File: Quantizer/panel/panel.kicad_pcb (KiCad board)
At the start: 2 copper layers, 50.8 x 128.5 mm, 13 parts

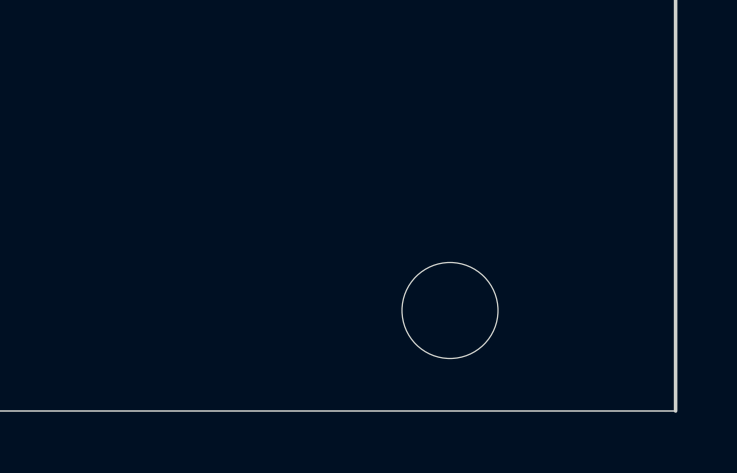
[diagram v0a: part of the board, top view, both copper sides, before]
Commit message: First commit
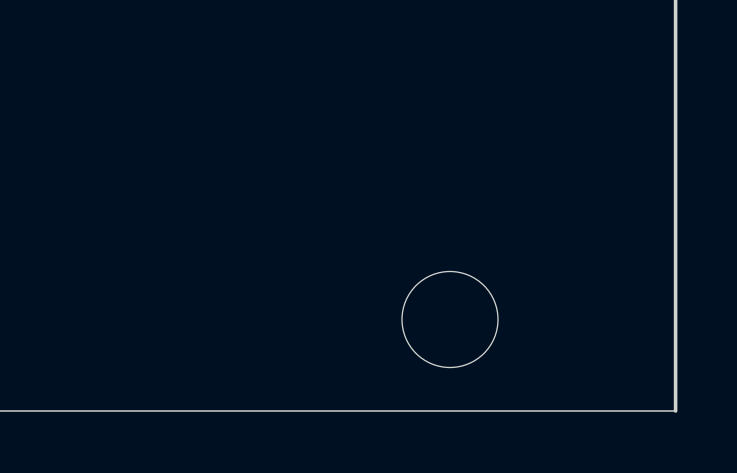
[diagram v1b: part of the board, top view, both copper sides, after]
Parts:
- moved H5 0.30 mm to (68.5, 153.3)
